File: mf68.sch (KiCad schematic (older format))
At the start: 2 parts, among them SW1 MX, U1 nice_nano

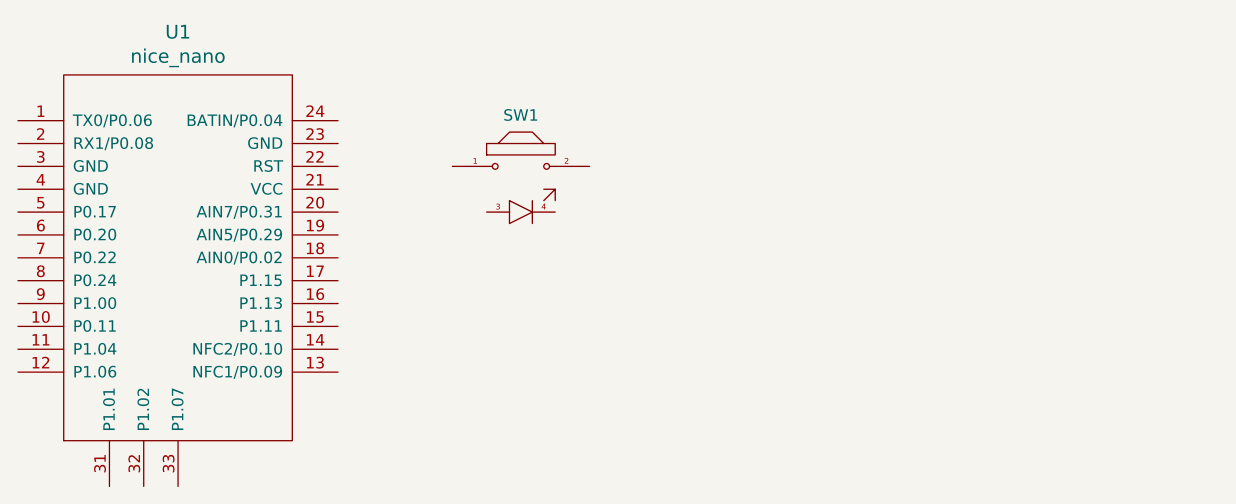
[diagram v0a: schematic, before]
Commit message: Start working on matrix
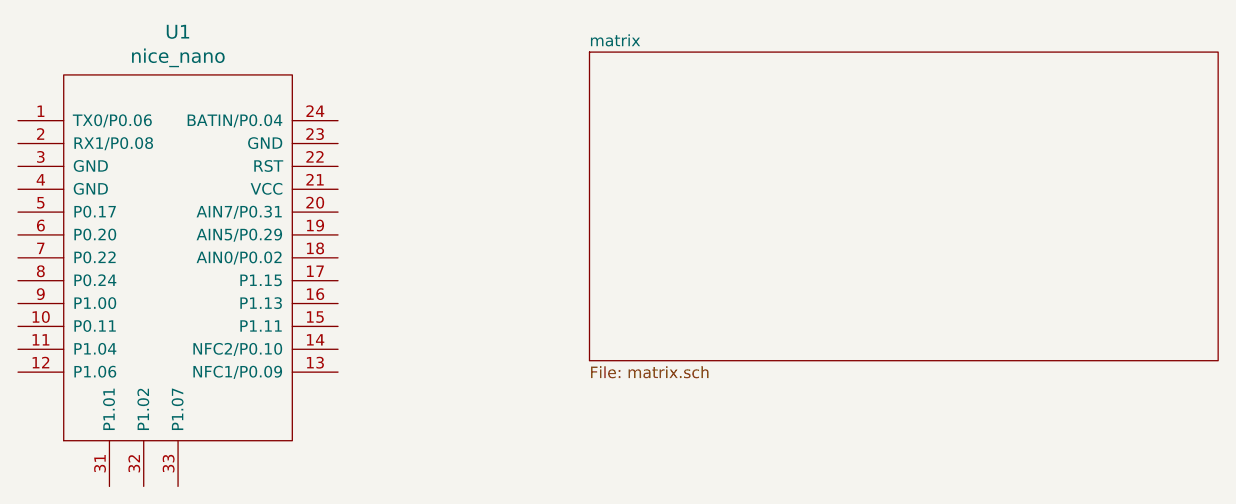
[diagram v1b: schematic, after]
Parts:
- removed SW1: MX, Keebio-Parts:MX-Alps-Choc-1U, symbol keebio:MX
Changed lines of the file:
@@
 $Descr A4 11693 8268
 encoding utf-8
-Sheet 1 1
+Sheet 1 2
 Title ""
 Date ""
@@
 	1    0    0    -1
 $EndComp
-$Comp
-L keebio:MX SW1
-U 1 1 6192757C
-P 3650 2550
-F 0 "SW1" H 3650 2773 50  0000 C CNN
-F 1 "MX" H 3650 2250 60  0001 C CNN
-F 2 "Keebio-Parts:MX-Alps-Choc-1U" H 3650 2550 60  0001 C CNN
-F 3 "" H 3650 2550 60  0001 C CNN
-	1    3650 2550
-	1    0    0    -1
-$EndComp
+$Sheet
+S 3950 2050 2750 1350
+U 6194AF7C
+F0 "matrix" 50
+F1 "matrix.sch" 50
+$EndSheet
 $EndSCHEMATC
